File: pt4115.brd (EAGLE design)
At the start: 14.6 x 17.1 mm, 6 parts

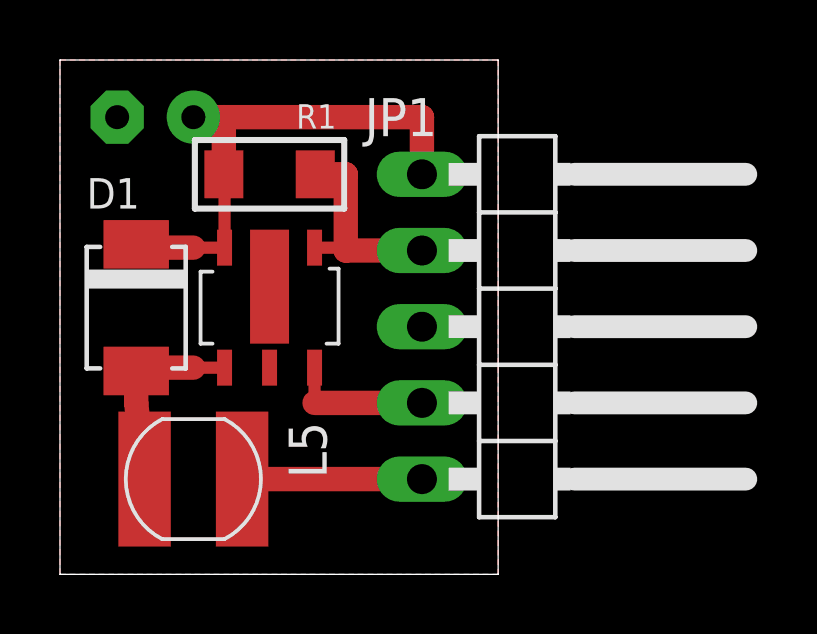
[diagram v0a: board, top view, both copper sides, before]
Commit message: pt4115 fixes
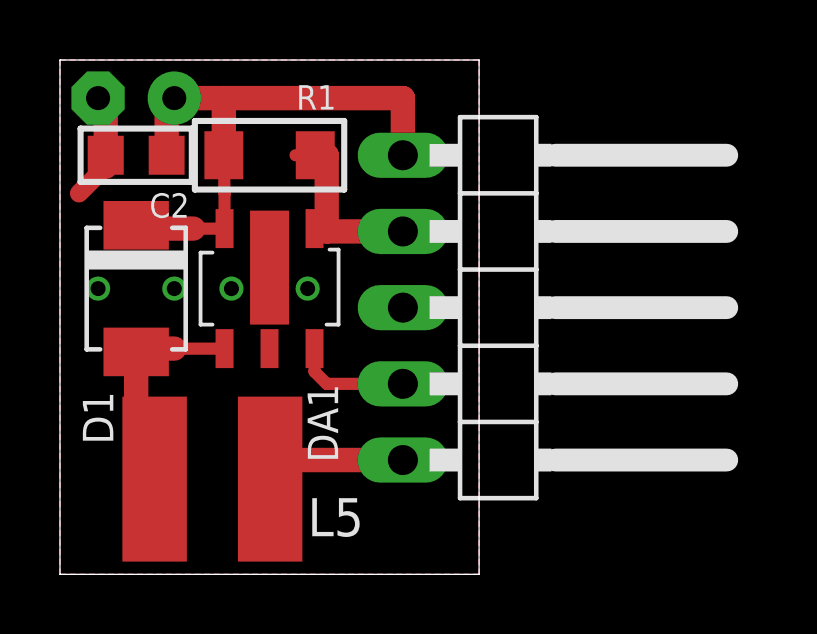
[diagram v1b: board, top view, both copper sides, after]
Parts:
- removed U$13: PT4115, 1dah:SOT89-5
- added C2: 0.1, rc-master-smd:C0805
- added DA1: PT4115, pt4115:SOT89-5
- L5: device rc-master-smd:CD43 -> rc-master-smd:CD54
- moved C1 0.90 mm to (2.54, 15.9)
- moved JP1 0.90 mm to (15.2, 8.89)
- moved D1 0.63 mm to (2.54, 9.53)
- moved L5 0.63 mm to (5.08, 3.17)
- moved R1 0.63 mm to (6.99, 14.0)
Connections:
- net GND: now also C2.2, DA1.2, DA1.PAD; no longer U$13.2, U$13.PAD
- net N$1: now also DA1.4; no longer U$13.4
- net N$3: now also DA1.3; no longer U$13.3
- net SW4: now also DA1.1; no longer U$13.1
- net V+: now also C2.1, DA1.5; no longer U$13.5
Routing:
- net GND: track 0.00 -> 3.65 mm, vias 0 -> 4
- net N$2: track 5.99 -> 4.73 mm
- net N$3: track 4.75 -> 3.88 mm
- net V+: track 18.1 -> 18.9 mm
- net N$1: track 7.16 -> 6.53 mm
- added copper zone on layer 16, net GND
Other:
- board size 14.6 x 17.1 mm -> 14 x 17.1 mm
